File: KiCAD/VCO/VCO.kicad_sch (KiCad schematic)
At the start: 38 parts, among them J1 AudioJack2_Ground, J2 AudioJack2_Ground, J3 AudioJack2_Ground, J4 AudioJack2_Ground, J5 AudioJack2_Ground, Q1 NPN, T1 PNP, T2 NPN, U1 4069

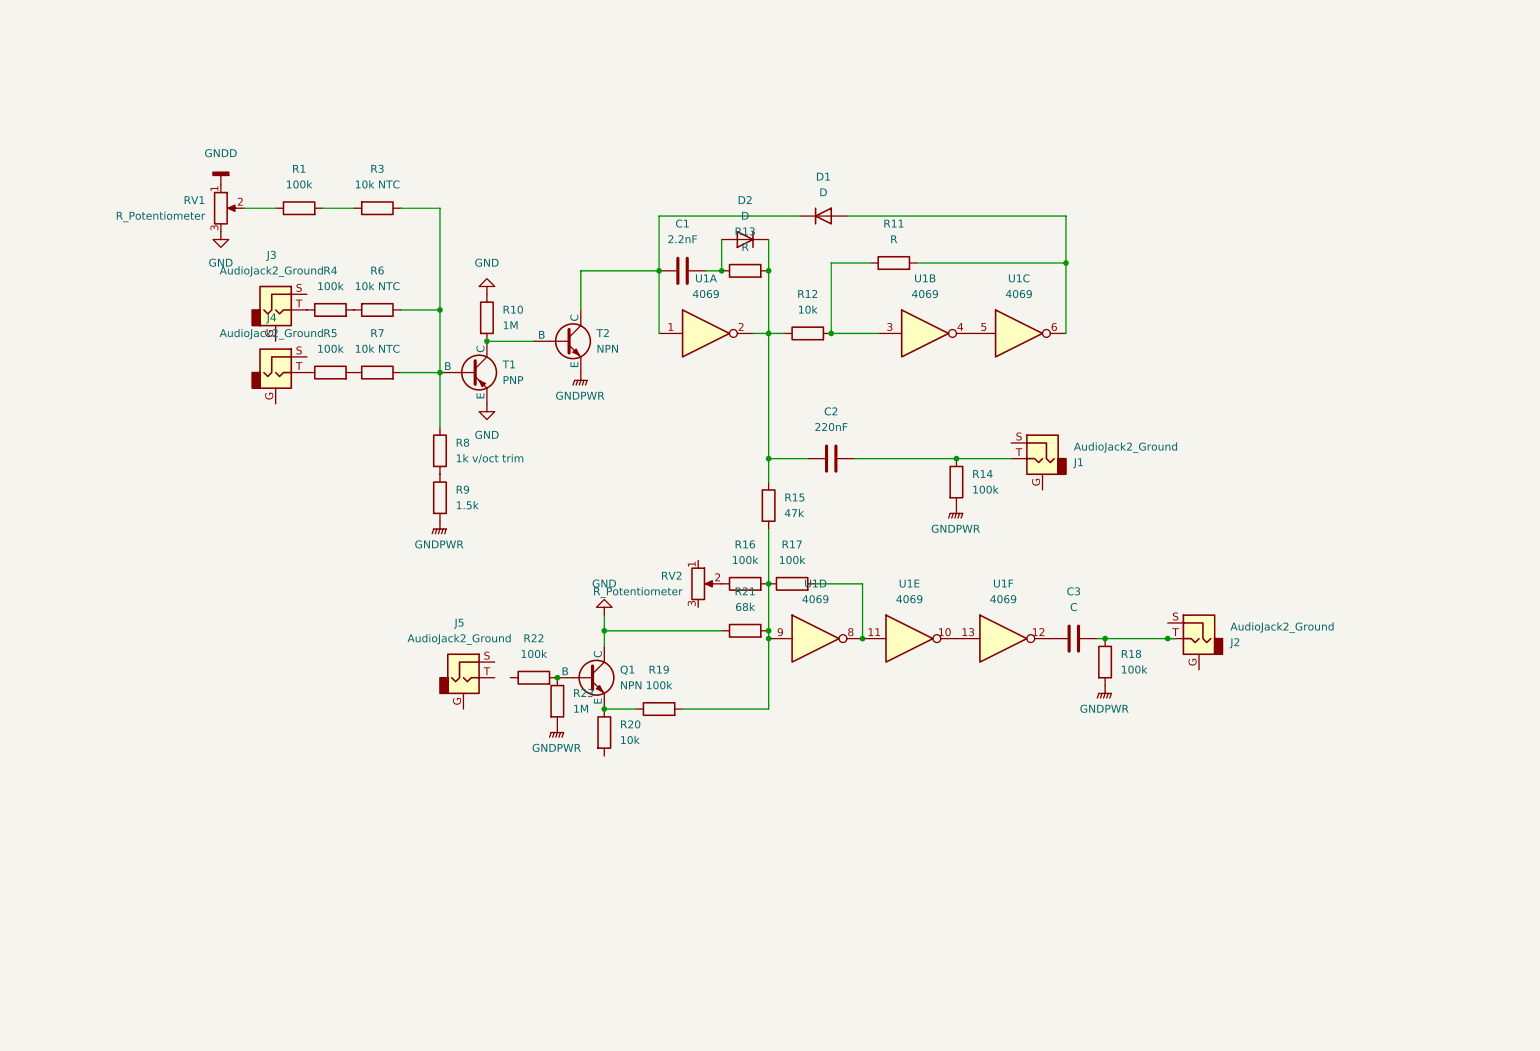
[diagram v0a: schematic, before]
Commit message: VCO and Power updates
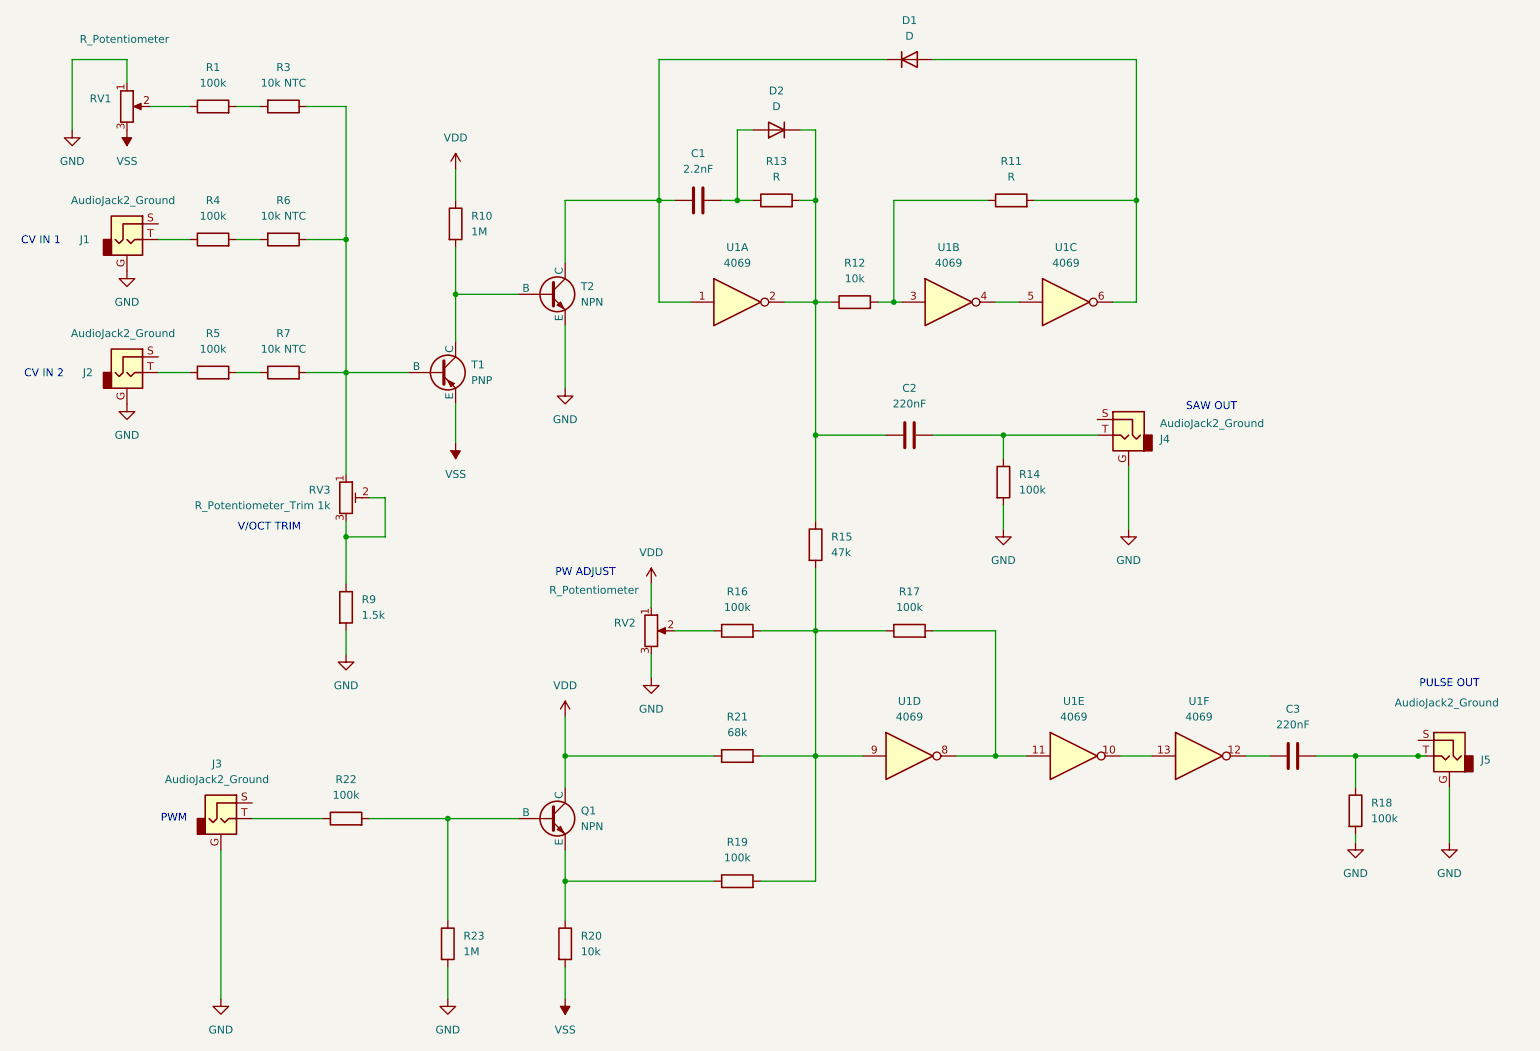
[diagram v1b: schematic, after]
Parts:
- removed R8: 1k v/oct trim, Resistor_THT:R_Axial_DIN0207_L6.3mm_D2.5mm_P7.62mm_Horizontal, symbol Device:R
- added RV3: R_Potentiometer_Trim 1k, symbol Device:R_Potentiometer_Trim
- C3: value C -> 220nF
- renumbered J3 to J1, J4 to J2, J5 to J3, J1 to J4, J2 to J5
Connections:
- net GNDD is gone; now on net GND: RV1.1
- net GNDPWR is gone; now on net GND: R14.2, R18.2, R23.2, R9.2, T2.3 (E)
- net GND: now also J1.G, J2.G, J3.G, J4.G, J5.G, RV2.3; no longer Q1.1 (C), R10.1, R21.1, RV1.3, T1.3 (E)
- net VDD: now reaches RV2.1
- net VDD: now also Q1.1 (C), R10.1, R21.1
- net at J3.T: now also R22.1
- net at R3.1, R6.1, R7.2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: now also RV3.1
- net at R9.1: now also RV3.2, RV3.3
- net VSS: now reaches R20.2
- net VSS: now also RV1.3, T1.3 (E)
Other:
- note added: "CV IN 1"
- note added: "CV IN 2"
- note added: "PULSE OUT"
- note added: "PW ADJUST"
- note added: "PWM"
- note added: "SAW OUT"
- note added: "V/OCT TRIM"
- moved on the sheet: C1, C2, C3, D1, D2, J1, J2, J3, J4, J5, Q1, R1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
